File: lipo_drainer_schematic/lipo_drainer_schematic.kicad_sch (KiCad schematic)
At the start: 58 parts, among them J1 BATT, J2 FAN, J3 Vcal, J4 128x64_OLED, J5 Gcal, J6 Ical, J7 Heatsink Temp (for MCP7901), Q1 MMBT3904, Q10 G700P06T, Q11 G700P06T, Q2 IRLML5103TRPBF, Q3 SiA469DJ, Q4 MMBT3904, Q5 IRLML5103TRPBF, Q6 MMBT3904, Q7 G700P06T, Q8 G700P06T, Q9 MMBT3904, SW1 OFF, SW2 NEXT, SW3 OK, SW4 RUN, SW5 ON, U2 Pico, U3 TPS70933DBVR, U4 LM4040DBZ-3, U5 LM4040DBZ-3

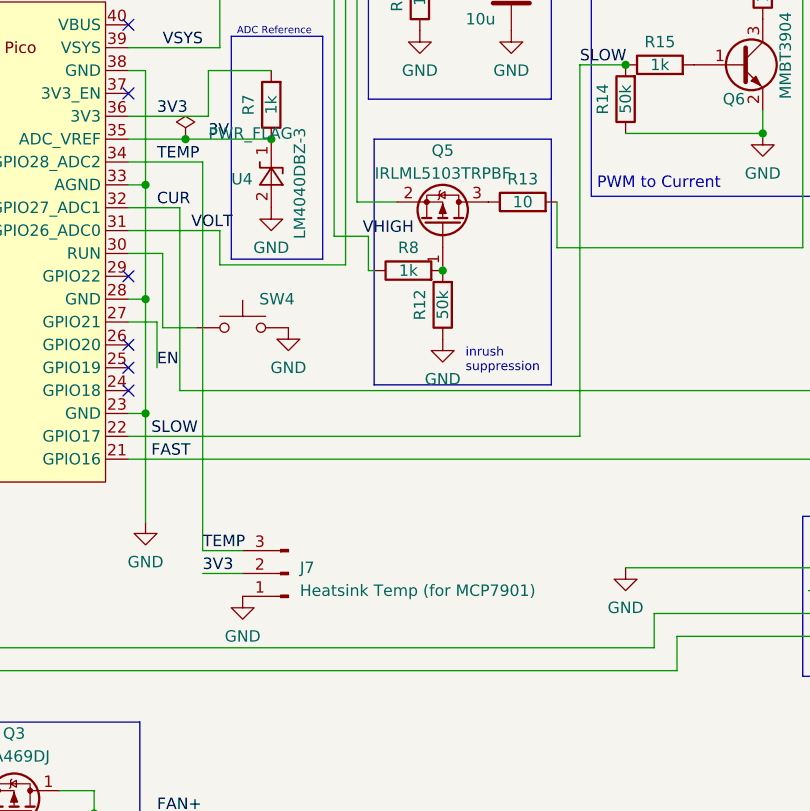
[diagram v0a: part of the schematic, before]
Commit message: Label cleanup
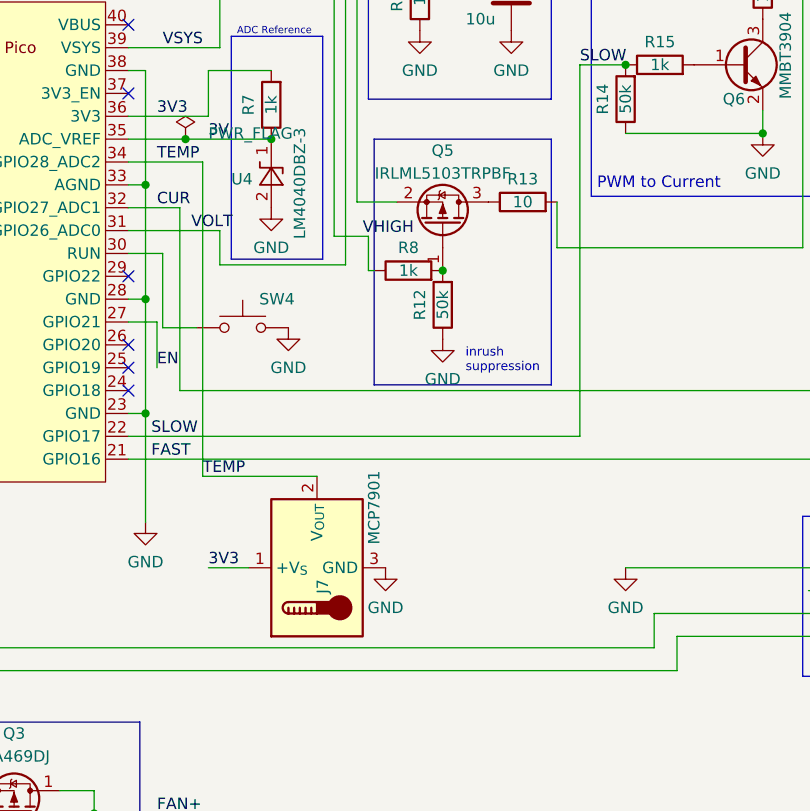
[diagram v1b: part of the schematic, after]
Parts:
- J7: value Heatsink Temp (for MCP7901) -> MCP7901; footprint Connector_PinHeader_2.54mm:PinHeader_1x03_P2.54mm_Vertical -> Package_TO_SOT_THT:TO-92_Inline; symbol Connector:Conn_01x03_Pin -> Sensor_Temperature:LM35-LP
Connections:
- net 3V3: now also J7.1 (+V_{S}); no longer J7.2 (Pin_2)
- net GND: now also J7.3 (GND); no longer J7.1 (Pin_1)
- net TEMP: now also J7.2 (V_{OUT}); no longer J7.3 (Pin_3)
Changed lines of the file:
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@@
     (stroke (width 0) (type default))
   )
-  (wire (pts (xy 150.495 90.17) (xy 150.495 133.35))
+  (wire (pts (xy 150.495 90.17) (xy 150.495 125.095))
     (stroke (width 0) (type default))
   )
@@
     (stroke (width 0) (type default))
   )
-  (wire (pts (xy 150.495 135.89) (xy 154.94 135.89))
+  (wire (pts (xy 151.13 135.255) (xy 155.575 135.255))
     (stroke (width 0) (type default))
   )
@@
     (stroke (width 0) (type default))
   )
+  (wire (pts (xy 101.6 144.145) (xy 200.66 144.145))
+    (stroke (width 0) (type default))
+  )
   (polyline (pts (xy 255.27 64.77) (xy 255.27 71.755))
     (stroke (width 0) (type default))
@@
     (stroke (width 0) (type default))
   )
-  (wire (pts (xy 101.6 144.145) (xy 200.66 144.145))
-    (stroke (width 0) (type default))
-  )
   (wire (pts (xy 71.755 55.88) (xy 76.835 55.88))
     (stroke (width 0) (type default))
@@
     (stroke (width 0) (type default))
   )
-  (wire (pts (xy 150.495 133.35) (xy 154.94 133.35))
+  (wire (pts (xy 150.495 125.095) (xy 163.195 125.095))
     (stroke (width 0) (type default))
   )
@@
     (effects (font (size 1.27 1.27)) (justify left bottom))
   )
-  (label "TEMP" (at 150.495 133.35 0) (fields_autoplaced)
+  (label "TEMP" (at 150.495 125.095 0) (fields_autoplaced)
     (effects (font (size 1.27 1.27)) (justify left bottom))
   )
@@
     (effects (font (size 1.27 1.27)) (justify left bottom))
   )
-  (label "3V3" (at 150.495 135.89 0) (fields_autoplaced)
+  (label "3V3" (at 151.13 135.255 0) (fields_autoplaced)
     (effects (font (size 1.27 1.27)) (justify left bottom))
   )
@@
     )
   )
-  (symbol (lib_id "Connector:Conn_01x03_Pin") (at 160.02 135.89 180) (unit 1)
-    (in_bom yes) (on_board yes) (dnp no) (fields_autoplaced)
-    (property "Reference" "J7" (at 161.29 135.255 0)
+  (symbol (lib_id "Sensor_Temperature:LM35-LP") (at 163.195 135.255 90) (unit 1)
+    (in_bom yes) (on_board yes) (dnp no)
+    (property "Reference" "J7" (at 163.83 136.525 0)
       (effects (font (size 1.27 1.27)) (justify right))
     )
-    (property "Value" "Heatsink Temp (for MCP7901)" (at 161.29 137.795 0)
+    (property "Value" "MCP7901" (at 169.545 124.46 0)
       (effects (font (size 1.27 1.27)) (justify right))
     )
-    (property "Footprint" "Connector_PinHeader_2.54mm:PinHeader_1x03_P2.54mm_Vertical" (at 160.02 135.89 0)
-      (effects (font (size 1.27 1.27)) hide)
-    )
-    (property "Datasheet" "~" (at 160.02 135.89 0)
+    (property "Footprint" "Package_TO_SOT_THT:TO-92_Inline" (at 169.545 133.985 0)
+      (effects (font (size 1.27 1.27)) (justify left) hide)
+    )
+    (property "Datasheet" "http://www.ti.com/lit/ds/symlink/lm35.pdf" (at 163.195 135.255 0)
       (effects (font (size 1.27 1.27)) hide)
     )
@@
     )
   )
-  (symbol (lib_id "power:GND") (at 154.94 138.43 0) (unit 1)
+  (symbol (lib_id "power:GND") (at 170.815 135.255 0) (unit 1)
     (in_bom yes) (on_board yes) (dnp no) (fields_autoplaced)
-    (property "Reference" "#PWR026" (at 154.94 144.78 0)
-      (effects (font (size 1.27 1.27)) hide)
-    )
-    (property "Value" "GND" (at 154.94 142.875 0)
-      (effects (font (size 1.27 1.27)))
-    )
-    (property "Footprint" "" (at 154.94 138.43 0)
-      (effects (font (size 1.27 1.27)) hide)
-    )
-    (property "Datasheet" "" (at 154.94 138.43 0)
-      (effects (font (size 1.27 1.27)) hide)
-    )
+    (property "Reference" "#PWR026" (at 170.815 141.605 0)
+      (effects (font (size 1.27 1.27)) hide)
+    )
+    (property "Value" "GND" (at 170.815 139.7 0)
+      (effects (font (size 1.27 1.27)))
+    )
+    (property "Footprint" "" (at 170.815 135.255 0)
+      (effects (font (size 1.27 1.27)) hide)
+    )
+    (property "Datasheet" "" (at 170.815 135.255 0)
+      (effects (font (size 1.27 1.27)) hide)
+    )
